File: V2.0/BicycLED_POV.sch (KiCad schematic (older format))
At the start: 57 parts, among them IC1 AT45DBXX1, IC2 AT91SAM7S512/256/128/64/321-AU, P1 CONN_2, Q1 BSH207, Q2 BSH207, Q3 2N2002K, SW1 bootloader, U1 CONN_MICROSD, U2 MCP73811/2, U3 CONN_JTAG_ARM, U4 USBCONN, U5 AH173, U6 FAN2502-XX, X1 18.432 MHz

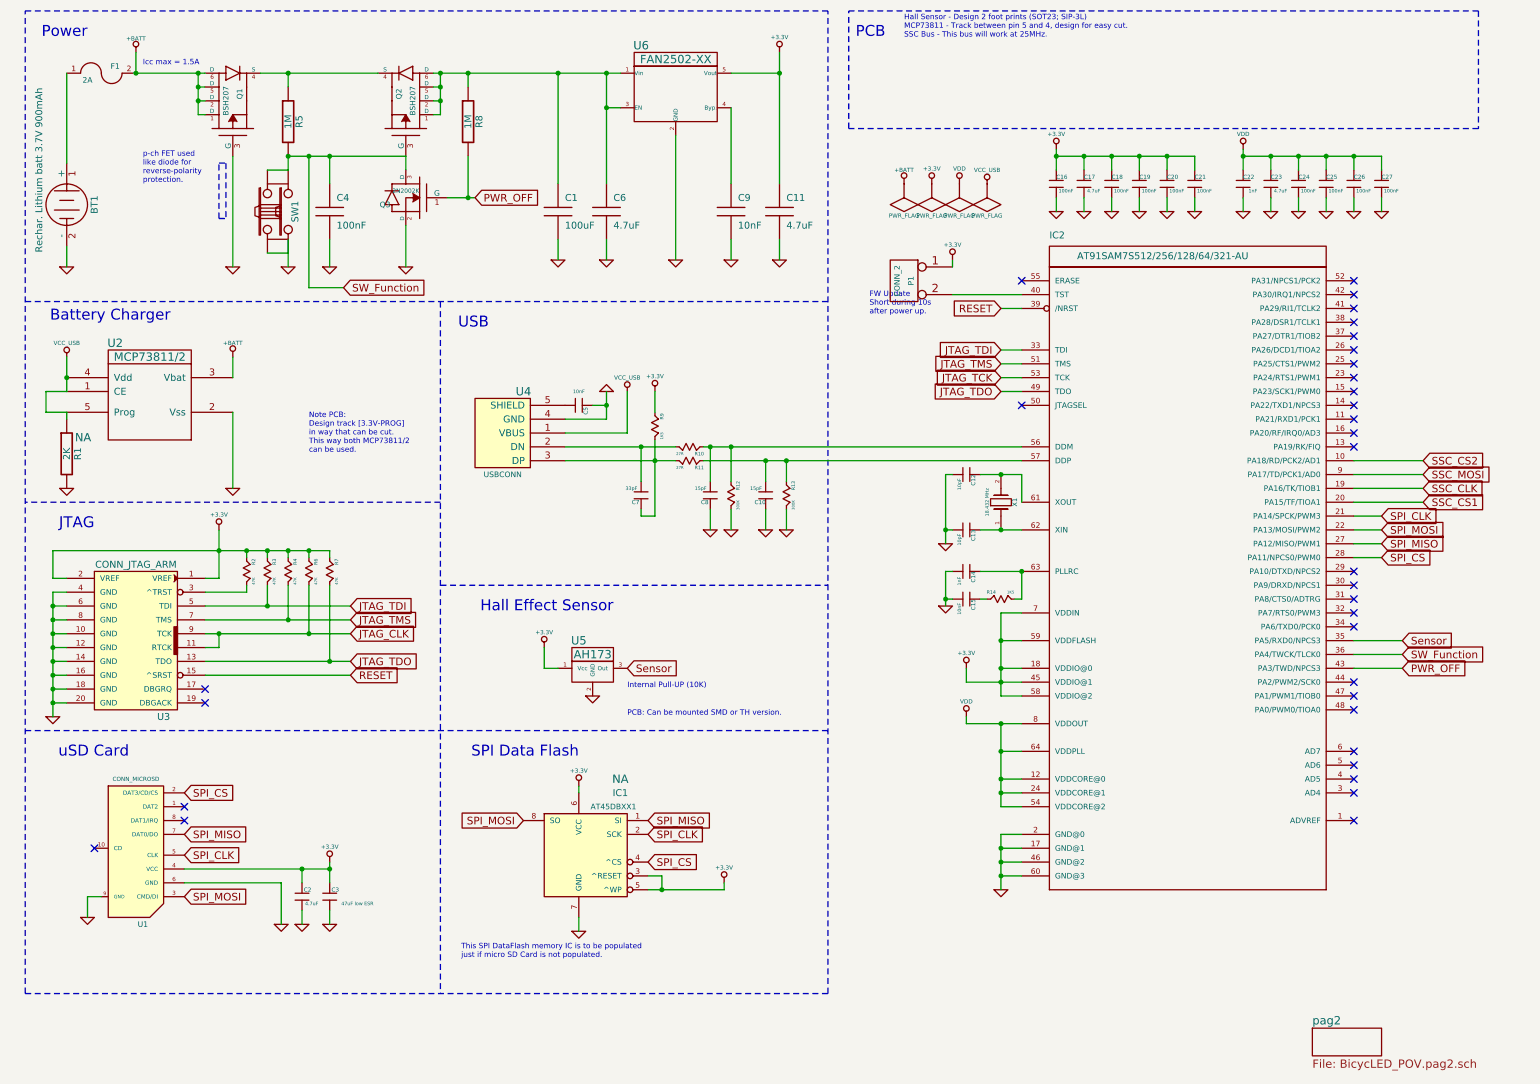
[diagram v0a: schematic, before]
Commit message: brd: created
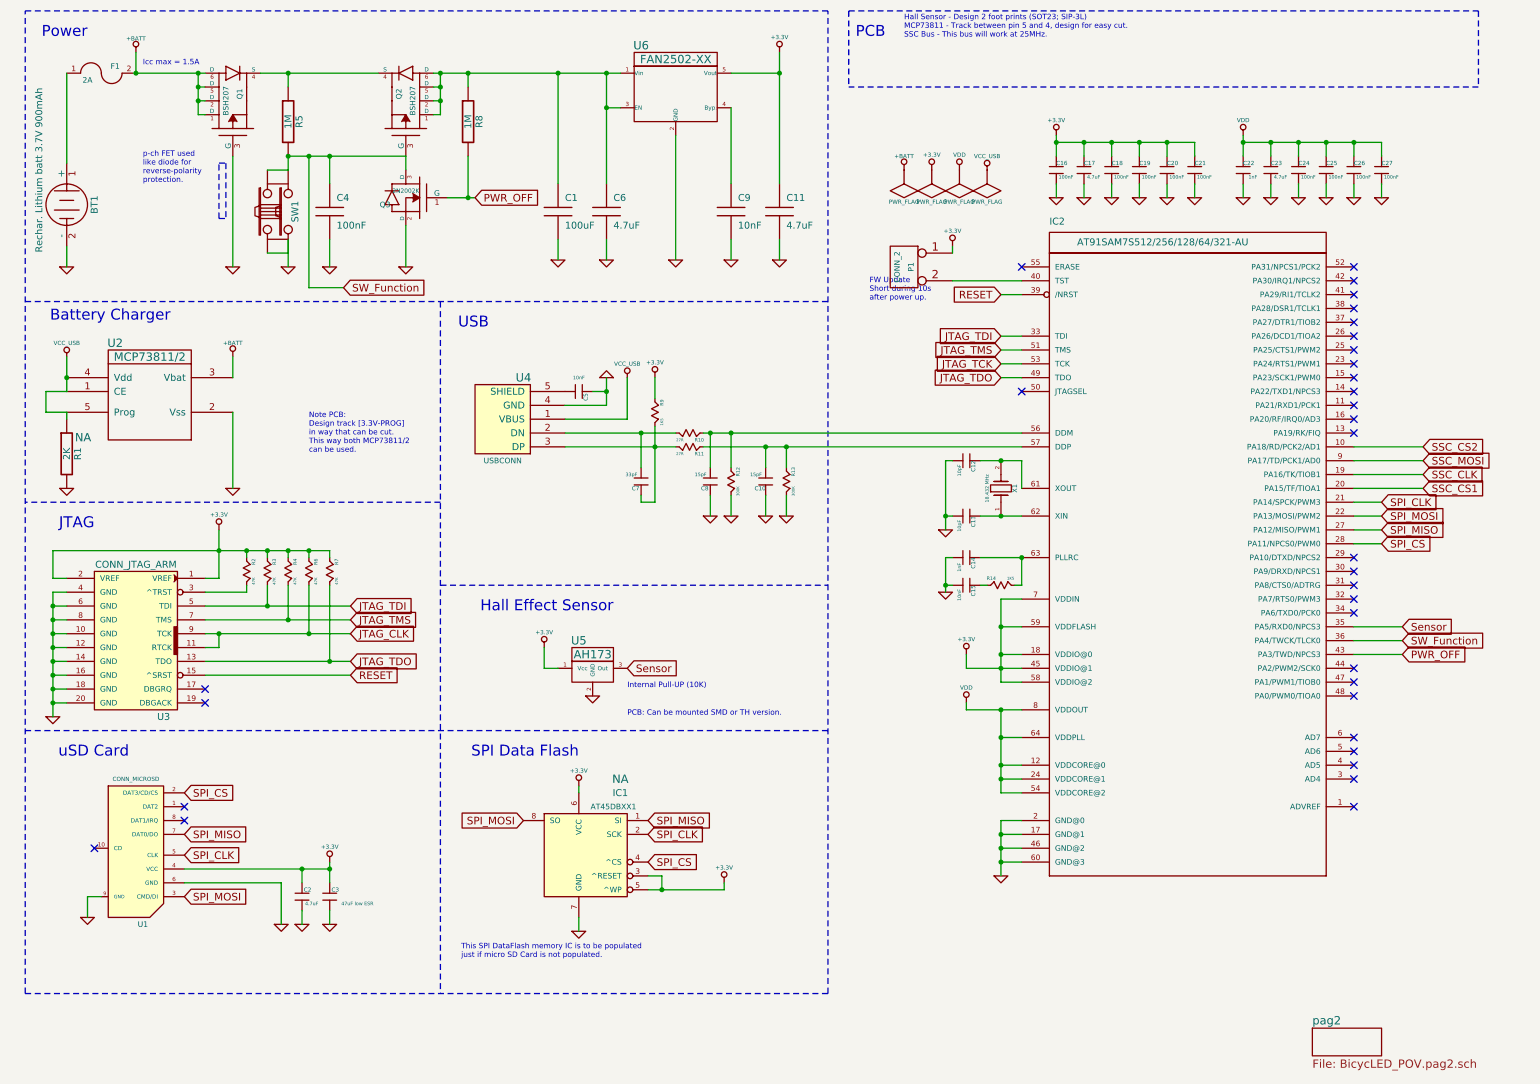
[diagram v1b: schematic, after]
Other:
- moved on the sheet: C10, C12, C13, C14, C15, C16, C17, C18, C19, C20, C21, C22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
